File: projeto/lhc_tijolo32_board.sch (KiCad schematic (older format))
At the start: 46 parts, among them J1 USB_A, J2 OLED, J3 JTAG 10pin Connector, J4 CONN_06POLAR, J5 CONN_06POLAR, Q1 MMBT3904, Q2 MMBT3904, SW1 SW_Push, SW2 SW_Push, U1 AP2112K-3.3, U2 CH340G, U3 ESP32-WROOM-32D, U4 AP2112K-3.3, Y1 12MHz 10ppm, Y2 32k 20ppm

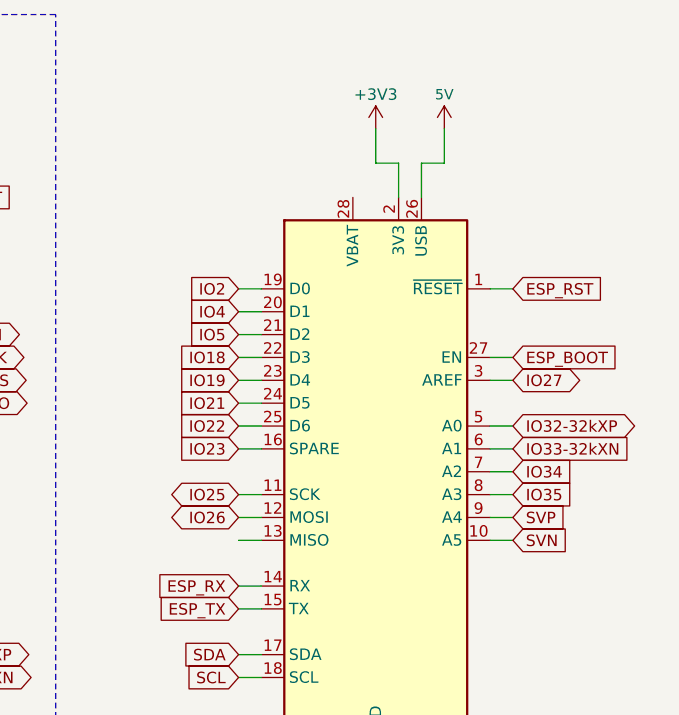
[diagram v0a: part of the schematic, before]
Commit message: Layout improved
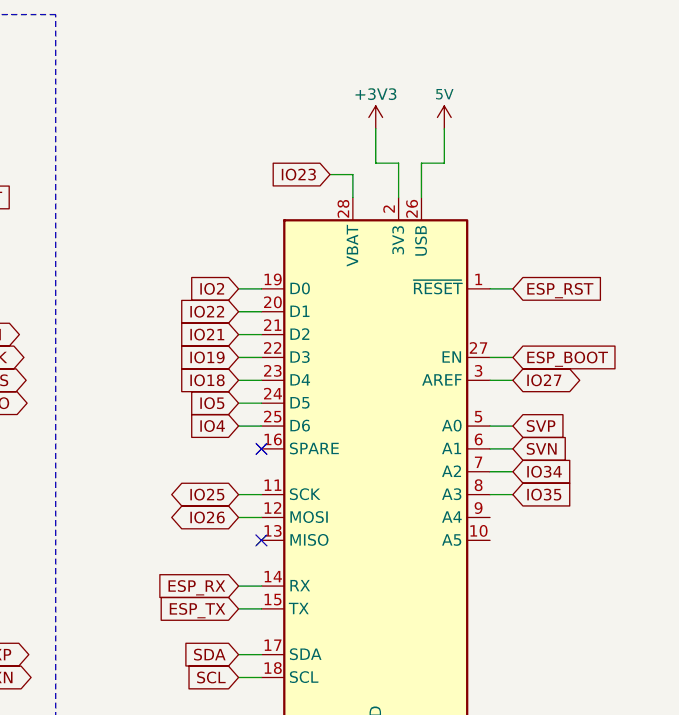
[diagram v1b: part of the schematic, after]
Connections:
- wire segments 255 -> 253
- no-connect marks 5 -> 7
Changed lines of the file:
@@
 Wire Notes Line
 	6350 3200 4750 3200
-Text GLabel 10600 2350 2    50   BiDi ~ 0
-IO32-32kXP
-Text GLabel 10600 2450 2    50   Input ~ 0
-IO33-32kXN
 Text GLabel 10600 2550 2    50   Input ~ 0
 IO34
@@
 Text GLabel 10600 1750 2    50   Input ~ 0
 ESP_RST
-Text GLabel 9400 2250 0    50   Input ~ 0
+Text GLabel 9400 1950 0    50   Input ~ 0
 IO21
 Text GLabel 9400 3150 0    50   Input ~ 0
@@
 Text GLabel 9400 3050 0    50   Input ~ 0
 ESP_RX
-Text GLabel 9400 2350 0    50   Input ~ 0
-IO22
+Text GLabel 9400 2050 0    50   Input ~ 0
+IO19
+Text GLabel 9800 1250 0    50   Input ~ 0
+IO23
 Text GLabel 9400 2150 0    50   Input ~ 0
-IO19
-Text GLabel 9400 2450 0    50   Input ~ 0
-IO23
-Text GLabel 9400 2050 0    50   Input ~ 0
 IO18
-Text GLabel 9400 1950 0    50   Input ~ 0
+Text GLabel 9400 2250 0    50   Input ~ 0
 IO5
 Text GLabel 9400 1750 0    50   Input ~ 0
@@
 Text GLabel 10600 2050 2    50   Input ~ 0
 ESP_BOOT
-Text GLabel 9400 1850 0    50   Input ~ 0
+Text GLabel 9400 2350 0    50   Input ~ 0
 IO4
 Text GLabel 9400 3350 0    50   Input ~ 0
@@
 	1    0    0    -1
 $EndComp
-Text GLabel 10600 2750 2    50   Input ~ 0
+Text GLabel 10600 2350 2    50   Input ~ 0
 SVP
-Text GLabel 10600 2850 2    50   Input ~ 0
+Text GLabel 10600 2450 2    50   Input ~ 0
 SVN
 $Comp
@@
 	9400 2350 9500 2350
 Wire Wire Line
-	9400 2450 9500 2450
-Wire Wire Line
 	10500 2350 10600 2350
 Wire Wire Line
@@
 	10500 2650 10600 2650
 Wire Wire Line
-	10500 2750 10600 2750
-Wire Wire Line
-	10500 2850 10600 2850
-Wire Wire Line
 	9400 2650 9500 2650
 Wire Wire Line
 	9400 2750 9500 2750
-Wire Wire Line
-	9400 2850 9500 2850
 Wire Wire Line
 	10000 3950 10000 3850
@@
 Wire Wire Line
 	10500 2150 10600 2150
+Text GLabel 9400 1850 0    50   Input ~ 0
+IO22
+Wire Wire Line
+	9800 1250 9900 1250
+Wire Wire Line
+	9900 1250 9900 1350
+NoConn ~ 9500 2450
+NoConn ~ 9500 2850
 $EndSCHEMATC

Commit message: Layout LIVE
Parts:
- JP1, JP2: footprint Jumper:SolderJumper-3_P1.3mm_Bridged12_Pad1.0x1.5mm_NumberLabels -> Jumper:SolderJumper-3_P1.3mm_Open_Pad1.0x1.5mm_NumberLabels; symbol Jumper:SolderJumper_3_Bridged12 -> Jumper:SolderJumper_3_Open
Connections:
- no-connect marks 7 -> 9
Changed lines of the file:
@@
 SDA
 $Comp
-L Jumper:SolderJumper_3_Bridged12 JP2
+L Jumper:SolderJumper_3_Open JP2
 U 1 1 5F71E23B
 P 3800 3850
 F 0 "JP2" H 3800 4055 50  0000 C CNN
 F 1 "P1" H 3800 3964 50  0000 C CNN
-F 2 "Jumper:SolderJumper-3_P1.3mm_Bridged12_Pad1.0x1.5mm_NumberLabels" H 3800 3850 50  0001 C CNN
+F 2 "Jumper:SolderJumper-3_P1.3mm_Open_Pad1.0x1.5mm_NumberLabels" H 3800 3850 50  0001 C CNN
 F 3 "~" H 3800 3850 50  0001 C CNN
 	1    3800 3850
@@
 $EndComp
 $Comp
-L Jumper:SolderJumper_3_Bridged12 JP1
+L Jumper:SolderJumper_3_Open JP1
 U 1 1 5F71F2AF
 P 3100 3850
 F 0 "JP1" H 3100 4055 50  0000 C CNN
 F 1 "P2" H 3100 3964 50  0000 C CNN
-F 2 "Jumper:SolderJumper-3_P1.3mm_Bridged12_Pad1.0x1.5mm_NumberLabels" H 3100 3850 50  0001 C CNN
+F 2 "Jumper:SolderJumper-3_P1.3mm_Open_Pad1.0x1.5mm_NumberLabels" H 3100 3850 50  0001 C CNN
 F 3 "~" H 3100 3850 50  0001 C CNN
 	1    3100 3850
@@
 Text GLabel 10600 2650 2    50   Input ~ 0
 IO35
-Text GLabel 9400 2650 0    50   BiDi ~ 0
+Text GLabel 10600 2750 2    50   BiDi ~ 0
 IO25
-Text GLabel 9400 2750 0    50   BiDi ~ 0
+Text GLabel 10600 2850 2    50   BiDi ~ 0
 IO26
 Text GLabel 10600 2150 2    50   BiDi ~ 0
@@
 	10500 2650 10600 2650
 Wire Wire Line
-	9400 2650 9500 2650
-Wire Wire Line
-	9400 2750 9500 2750
-Wire Wire Line
 	10000 3950 10000 3850
 $Comp
@@
 NoConn ~ 9500 2450
 NoConn ~ 9500 2850
+Wire Wire Line
+	10500 2750 10600 2750
+Wire Wire Line
+	10500 2850 10600 2850
+NoConn ~ 9500 2750
+NoConn ~ 9500 2650
 $EndSCHEMATC
